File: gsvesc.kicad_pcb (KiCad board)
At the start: 4 copper layers, 115 x 115 mm, 125 parts, among them J1 Conn_01x06, J10 PHASE_C, J11 PHASE_A, J12 NTC, J13 PHASE_B, J14 Conn_02x04_Odd_Even, J2 Conn_01x06, J3 Conn_01x06, J4 Conn_01x05, J5 Conn_01x03, J6 USB_B_Mini, J7 BAT+, J8 BAT-, Q1 NVMFS5C604, Q2 NVMFS5C604, Q3 NVMFS5C604, Q4 NVMFS5C604, Q5 NVMFS5C604, Q6 NVMFS5C604, U1 STM32F405RGTx, U2 IRU1010-33, U3 DRV8301DCAR, U4 AD8418, U5 AD8418, U6 AD8418, U7 M74VHC1GT66DTT1G, U8 M74VHC1GT66DTT1G, U9 M74VHC1GT66DTT1G, Y1 ABM3B 8MHz

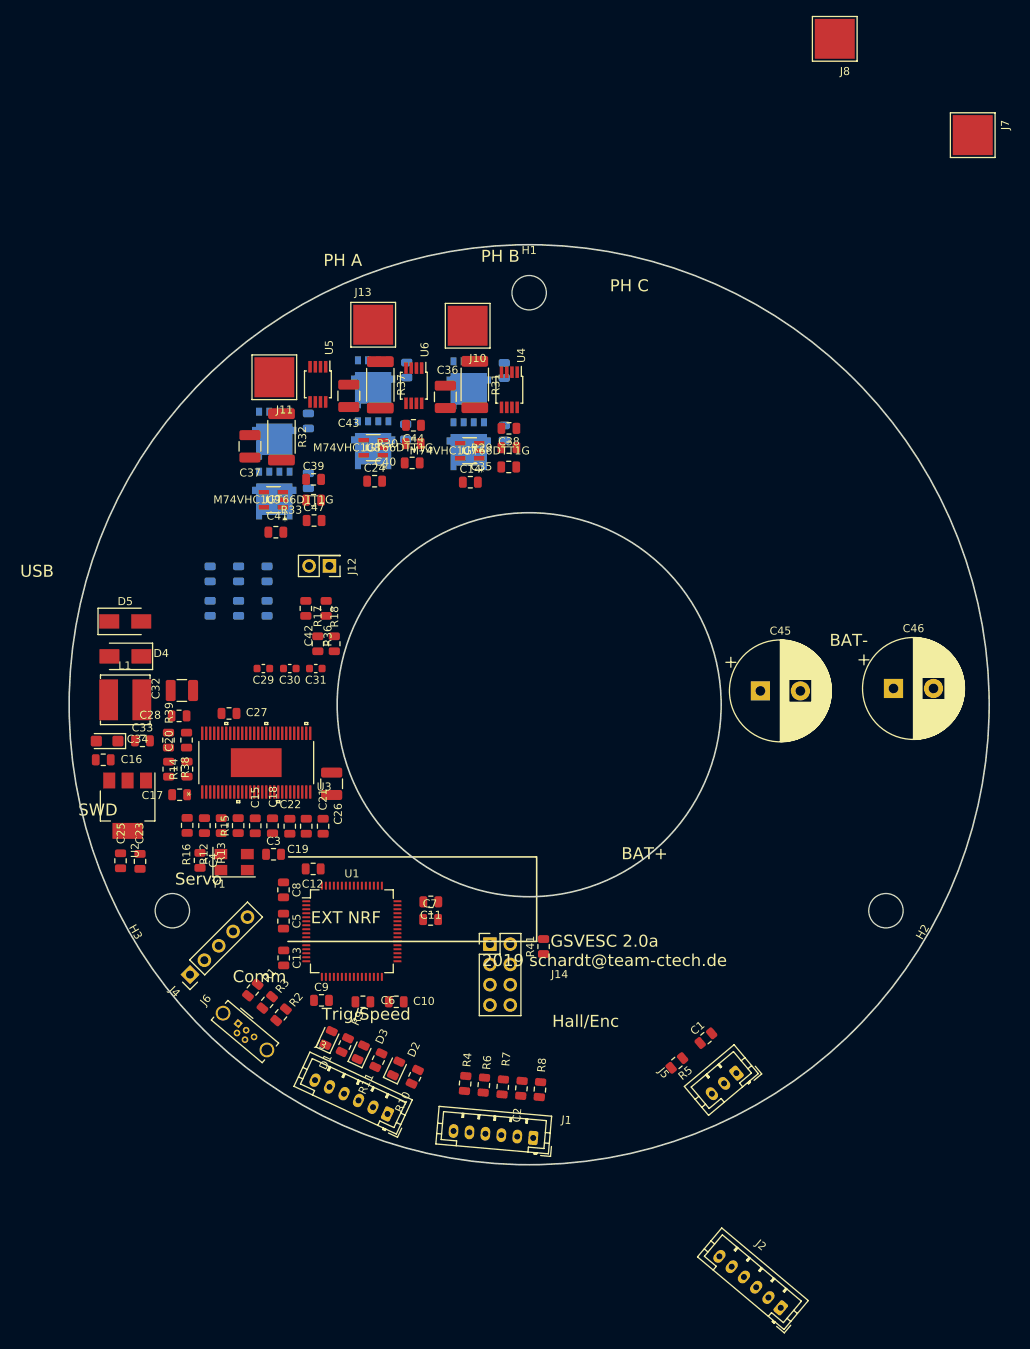
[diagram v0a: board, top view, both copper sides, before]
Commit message: Update
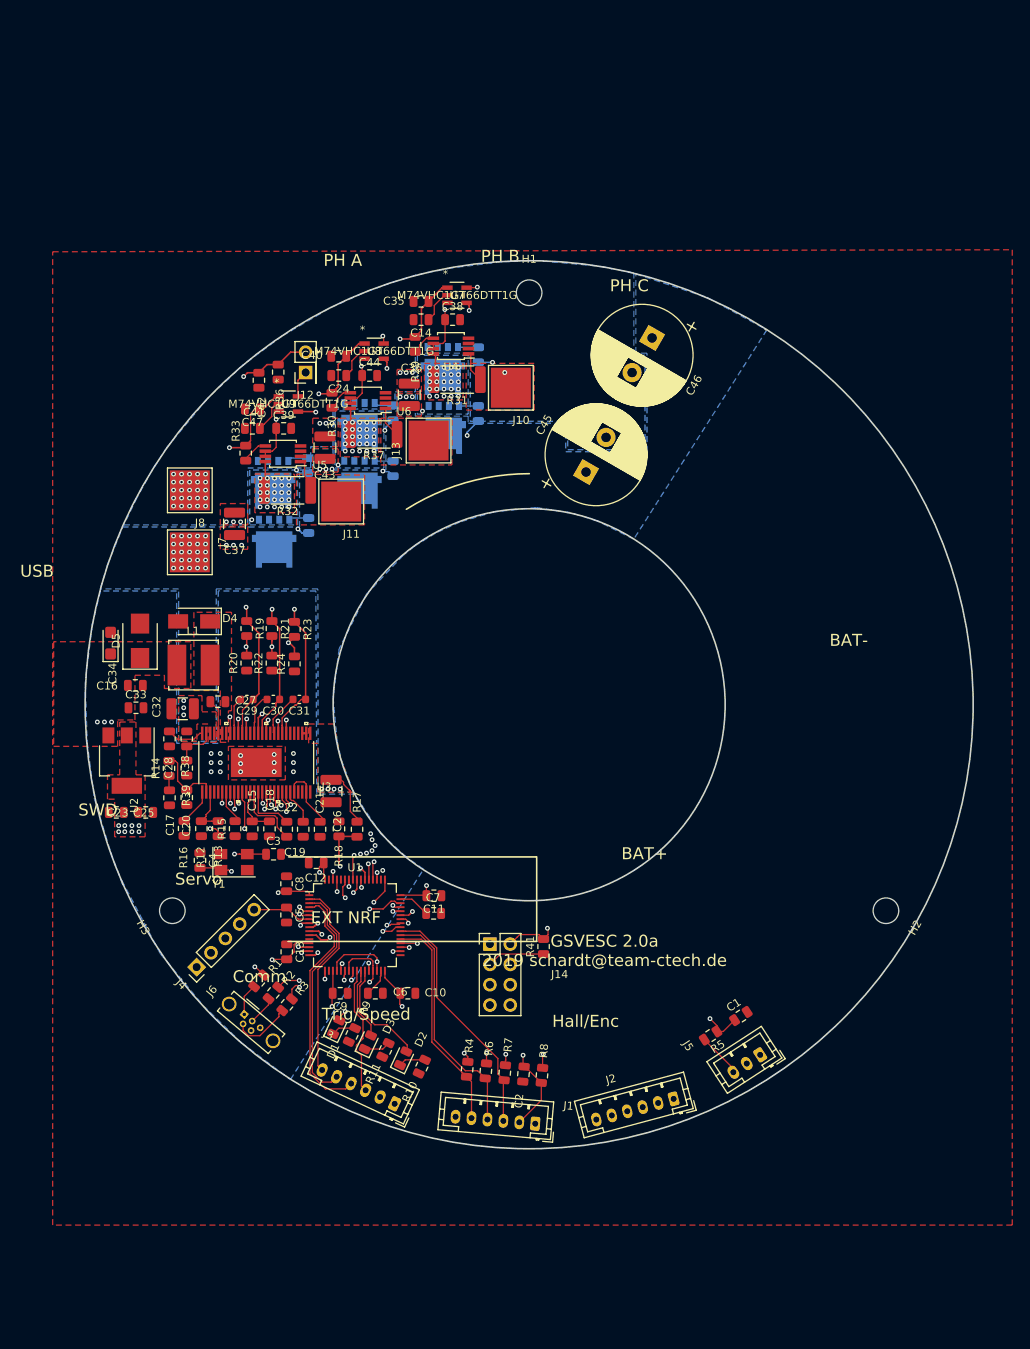
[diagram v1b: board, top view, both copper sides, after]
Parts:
- C26, C32: value 47u0/100V -> 10u0/100V
- C45, C46: value 680u/80V -> 680u/63V
- D5: value D -> SMBJ6.0CA; footprint Diode_SMD:D_SMA -> Diode_SMD:D_SMB
- H1, H2, H3: footprint MountingHole:MountingHole_4.3mm_M4 -> MountingHole:MountingHole_3.2mm_M3
- R19, R20, R21, R22, R23, R24: moved to F.Cu
- moved J7 110.9 mm to (57.6, 80.9)
- moved J8 98.4 mm to (57.6, 73.2)
- moved C46 53.2 mm to (115.4, 54.2), turned to 240 degrees
- moved C45 35.0 mm to (107.1, 70.9), turned to 60 degrees
- moved R36 30.1 mm to (68.6, 58.4)
- moved J2 29.4 mm to (118.1, 149.3), turned to 195 degrees
- moved C42 29.1 mm to (66.2, 59.4)
- moved J12 24.4 mm to (72.1, 58.5), turned to 90 degrees
- moved R17 23.7 mm to (78.5, 115.6)
- moved C35 23.4 mm to (86.5, 49.6)
- moved R18 23.2 mm to (76.2, 115.5), turned to 270 degrees
- moved C14 21.2 mm to (86.5, 51.9), turned to 180 degrees
- moved U7 19.5 mm to (91.0, 48.8), turned to 0 degrees
- moved J11 17.6 mm to (76.5, 74.6)
- moved R29 17.4 mm to (85.8, 55.0), turned to 90 degrees
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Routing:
- net /MCU/ADC_TEMP: track 0.00 -> 93.4 mm, vias 0 -> 2
- net /MCU/CURRENT_3: track 0.00 -> 93.2 mm, vias 0 -> 2
- net /POWER/CURR_FILTER: track 0.00 -> 91.1 mm, vias 0 -> 4
- net /MCU/CURRENT_2: track 0.00 -> 78.8 mm, vias 0 -> 2
- net /MCU/CURRENT_1: track 0.00 -> 75.8 mm, vias 0 -> 2
- net VCC: track 0.00 -> 67.5 mm, vias 0 -> 26
- net /MCU/SERVO: track 0.00 -> 60.8 mm, vias 0 -> 2
- net /DRV8301/GL_C: track 0.00 -> 58.8 mm, vias 0 -> 2
- net /DRV8301/SH_C: track 0.00 -> 50.9 mm, vias 0 -> 27
- net /DRV8301/GH_C: track 0.00 -> 50.0 mm, vias 0 -> 2
- net /MCU/RX_SDA_NSS: track 0.00 -> 49.0 mm, vias 0 -> 1
- net /DRV8301/SENS_C: track 0.00 -> 47.8 mm, vias 0 -> 2
- net /DRV8301/GL_B: track 0.00 -> 46.1 mm, vias 0 -> 2
- net /DRV8301/SENS_B: track 0.00 -> 45.5 mm, vias 0 -> 2
- net /MCU/SCK_ADC_EXT: track 0.00 -> 44.3 mm, vias 0 -> 1
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- added copper zone on B.Cu, net +5V
- added copper zone on F.Cu, net +5V
- added copper zone on B.Cu, net /DRV8301/SH_A
- added copper zone on F.Cu, net /DRV8301/SH_A
- added copper zone on In1.Cu, net /DRV8301/SH_A
- added copper zone on In2.Cu, net /DRV8301/SH_A
- added copper zone on B.Cu, net /DRV8301/SH_B
- added copper zone on F.Cu, net /DRV8301/SH_B
- added copper zone on In1.Cu, net /DRV8301/SH_B
- added copper zone on In2.Cu, net /DRV8301/SH_B
- added copper zone on B.Cu, net /DRV8301/SH_C
- added copper zone on F.Cu, net /DRV8301/SH_C
- added copper zone on In1.Cu, net /DRV8301/SH_C
- added copper zone on In2.Cu, net /DRV8301/SH_C
- added copper zone on B.Cu, net /DRV8301/VBAT
- added copper zone on F.Cu, net /DRV8301/VBAT
- added copper zone on In1.Cu, net /DRV8301/VBAT
- added copper zone on In2.Cu, net /DRV8301/VBAT
- added copper zone on F.Cu, net /POWER/PHASE_A
- added copper zone on F.Cu, net /POWER/PHASE_B
- added copper zone on F.Cu, net /POWER/PHASE_C
- added copper zone on B.Cu, net GND
- added copper zone on F.Cu, net GND
- added copper zone on In1.Cu, net GND
- added copper zone on In2.Cu, net GND
- added copper zone on F.Cu, net Net-(C27-Pad1)
- added copper zone on F.Cu, net VCC
- added copper zone on In2.Cu, net VCC
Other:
- board size 115 x 115 mm -> 111 x 111 mm
- net class Default: trace_width 0.2 -> 0.15
- net class POWER added: clearance 0.15, trace_width 0.2, via_dia 0.6, via_drill 0.3
